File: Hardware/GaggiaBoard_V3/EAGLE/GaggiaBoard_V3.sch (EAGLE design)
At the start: 73 parts, among them IC1 LD117AS33TR, J1 4PIN, J10 PIN262409-1, J11 PIN262409-1, J12 PIN262409-1, J13 PIN262409-1, J2 Vertical Qwiic Connector, J27 6PIN, J5 2PIN, J6 3PIN, J7 3PIN, J8 5PIN, J9 3PIN, K1 AQH213, Q10 600mA/40V, Q11 MOSFET_PCH_DUAL-DMP2240UDM, U1 BLACKPILL, U2 MAX31855K, U5 TXS0102

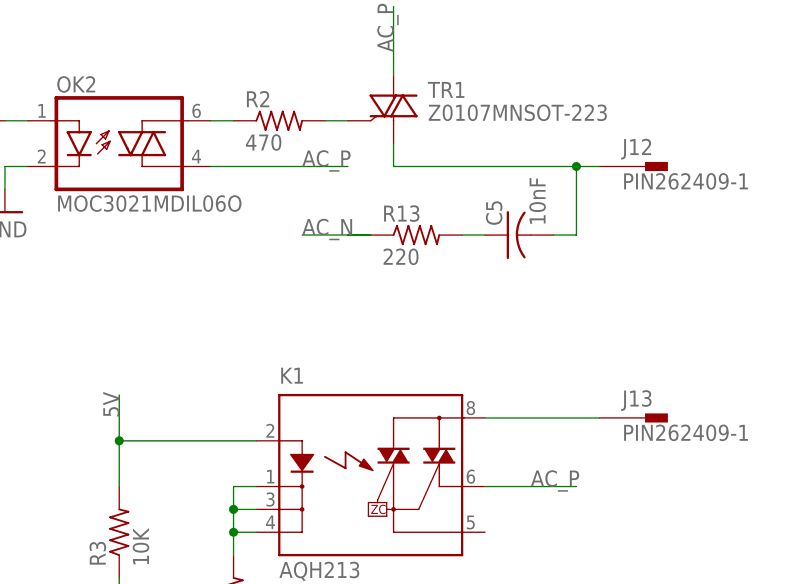
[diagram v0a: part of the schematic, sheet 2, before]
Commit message: snubbers
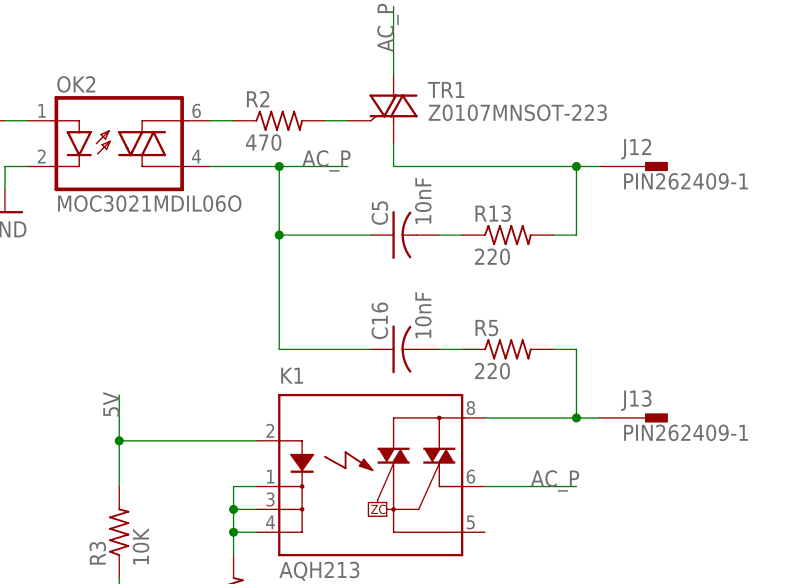
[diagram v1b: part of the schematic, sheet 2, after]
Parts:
- added C16: 10nF, rcl:C-USC1206
- added R5: 220, rcl:R-US_R2512
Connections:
- removed net N$32: C5.1, R13.2
- new net N$15: C16.2, R5.1
- new net N$16: C5.2, R13.1
- net 3WAY: now also R5.2
- net AC_N: no longer R13.1
- net AC_P: now also C16.1, C5.1
- net PUMP_P: now also R13.2; no longer C5.2
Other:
- moved on the sheet: C5, R13
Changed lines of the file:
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@@
 <attribute name="LCSC" value="C98220"/>
+</part>
+<part name="R5" library="rcl" library_urn="urn:adsk.eagle:library:334" deviceset="R-US_" device="R2512" package3d_urn="urn:adsk.eagle:package:23545/2" value="220">
+<spice>
+<pinmapping spiceprefix="R">
+<pinmap gate="G$1" pin="1" pinorder="1"/>
+<pinmap gate="G$1" pin="2" pinorder="2"/>
+</pinmapping>
+</spice>
+<attribute name="LCSC" value="C877859"/>
+</part>
+<part name="C16" library="rcl" library_urn="urn:adsk.eagle:library:334" deviceset="C-US" device="C1206" package3d_urn="urn:adsk.eagle:package:23618/2" value="10nF">
+<spice>
+<pinmapping spiceprefix="C">
+<pinmap gate="G$1" pin="1" pinorder="1"/>
+<pinmap gate="G$1" pin="2" pinorder="2"/>
+</pinmapping>
+</spice>
+<attribute name="LCSC" value="C107192"/>
 </part>
 </parts>
@@
 <instance part="MARK4" gate="G$1" x="243.84" y="27.94" smashed="yes"/>
 <instance part="MARK3" gate="G$1" x="241.3" y="27.94" smashed="yes"/>
-<instance part="R13" gate="G$1" x="208.28" y="109.22" smashed="yes">
-<attribute name="NAME" x="204.47" y="110.7186" size="1.778" layer="95"/>
-<attribute name="VALUE" x="204.47" y="105.918" size="1.778" layer="96"/>
-<attribute name="LCSC" x="208.28" y="109.22" size="1.778" layer="96" display="off"/>
-</instance>
-<instance part="C5" gate="G$1" x="218.44" y="109.22" smashed="yes" rot="R90">
-<attribute name="NAME" x="217.805" y="110.236" size="1.778" layer="95" rot="R90"/>
-<attribute name="VALUE" x="222.631" y="110.236" size="1.778" layer="96" rot="R90"/>
-<attribute name="LCSC" x="218.44" y="109.22" size="1.778" layer="96" rot="R90" display="off"/>
+<instance part="R13" gate="G$1" x="218.44" y="109.22" smashed="yes">
+<attribute name="NAME" x="214.63" y="110.7186" size="1.778" layer="95"/>
+<attribute name="VALUE" x="214.63" y="105.918" size="1.778" layer="96"/>
+<attribute name="LCSC" x="218.44" y="109.22" size="1.778" layer="96" display="off"/>
+</instance>
+<instance part="C5" gate="G$1" x="205.74" y="109.22" smashed="yes" rot="R90">
+<attribute name="NAME" x="205.105" y="110.236" size="1.778" layer="95" rot="R90"/>
+<attribute name="VALUE" x="209.931" y="110.236" size="1.778" layer="96" rot="R90"/>
+<attribute name="LCSC" x="205.74" y="109.22" size="1.778" layer="96" rot="R90" display="off"/>
 </instance>
 <instance part="MARK6" gate="G$1" x="238.76" y="27.94" smashed="yes"/>
@@
 <attribute name="LCSC" x="162.56" y="63.5" size="1.778" layer="96" display="off"/>
 </instance>
+<instance part="R5" gate="G$1" x="218.44" y="96.52" smashed="yes">
+<attribute name="NAME" x="214.63" y="98.0186" size="1.778" layer="95"/>
+<attribute name="VALUE" x="214.63" y="93.218" size="1.778" layer="96"/>
+<attribute name="LCSC" x="218.44" y="96.52" size="1.778" layer="96" display="off"/>
+</instance>
+<instance part="C16" gate="G$1" x="205.74" y="96.52" smashed="yes" rot="R90">
+<attribute name="NAME" x="205.105" y="97.536" size="1.778" layer="95" rot="R90"/>
+<attribute name="VALUE" x="209.931" y="97.536" size="1.778" layer="96" rot="R90"/>
+<attribute name="LCSC" x="205.74" y="96.52" size="1.778" layer="96" rot="R90" display="off"/>
+</instance>
 </instances>
 <busses>
@@
 </segment>
 <segment>
-<label x="195.58" y="109.22" size="1.778" layer="95"/>
-<pinref part="R13" gate="G$1" pin="1"/>
-<wire x1="203.2" y1="109.22" x2="200.66" y2="109.22" width="0.1524" layer="91"/>
-<wire x1="195.58" y1="109.22" x2="203.2" y2="109.22" width="0.1524" layer="91"/>
-</segment>
-<segment>
 <label x="5.08" y="68.58" size="1.778" layer="95"/>
 <wire x1="15.24" y1="68.58" x2="5.08" y2="68.58" width="0.1524" layer="91"/>
@@
 <segment>
 <pinref part="OK2" gate="G$1" pin="A1"/>
-<wire x1="185.42" y1="116.84" x2="200.66" y2="116.84" width="0.1524" layer="91"/>
+<wire x1="185.42" y1="116.84" x2="193.04" y2="116.84" width="0.1524" layer="91"/>
 <label x="195.58" y="116.84" size="1.778" layer="95"/>
+<pinref part="C5" gate="G$1" pin="1"/>
+<wire x1="193.04" y1="116.84" x2="200.66" y2="116.84" width="0.1524" layer="91"/>
+<wire x1="203.2" y1="109.22" x2="193.04" y2="109.22" width="0.1524" layer="91"/>
+<wire x1="193.04" y1="109.22" x2="193.04" y2="116.84" width="0.1524" layer="91"/>
+<junction x="193.04" y="116.84"/>
+<pinref part="C16" gate="G$1" pin="1"/>
+<wire x1="203.2" y1="96.52" x2="193.04" y2="96.52" width="0.1524" layer="91"/>
+<wire x1="193.04" y1="96.52" x2="193.04" y2="109.22" width="0.1524" layer="91"/>
+<junction x="193.04" y="109.22"/>
 </segment>
 <segment>
@@
 <net name="3WAY" class="0">
 <segment>
-<wire x1="228.6" y1="88.9" x2="215.9" y2="88.9" width="0.1524" layer="91"/>
+<wire x1="228.6" y1="88.9" x2="226.06" y2="88.9" width="0.1524" layer="91"/>
 <pinref part="J13" gate="-1" pin="1"/>
 <pinref part="K1" gate="G$1" pin="DS1"/>
+<pinref part="R5" gate="G$1" pin="2"/>
+<wire x1="226.06" y1="88.9" x2="215.9" y2="88.9" width="0.1524" layer="91"/>
+<wire x1="223.52" y1="96.52" x2="226.06" y2="96.52" width="0.1524" layer="91"/>
+<wire x1="226.06" y1="96.52" x2="226.06" y2="88.9" width="0.1524" layer="91"/>
+<junction x="226.06" y="88.9"/>
 </segment>
 </net>
@@
 </segment>
 </net>
-<net name="N$32" class="0">
-<segment>
-<pinref part="C5" gate="G$1" pin="1"/>
-<pinref part="R13" gate="G$1" pin="2"/>
-<wire x1="215.9" y1="109.22" x2="213.36" y2="109.22" width="0.1524" layer="91"/>
-</segment>
-</net>
 <net name="PUMP_P" class="0">
 <segment>
 <pinref part="J12" gate="-1" pin="1"/>
 <wire x1="228.6" y1="116.84" x2="226.06" y2="116.84" width="0.1524" layer="91"/>
+<pinref part="TR1" gate="G$1" pin="A1"/>
 <wire x1="226.06" y1="116.84" x2="205.74" y2="116.84" width="0.1524" layer="91"/>
-<pinref part="C5" gate="G$1" pin="2"/>
+<wire x1="205.74" y1="116.84" x2="205.74" y2="119.38" width="0.1524" layer="91"/>
+<pinref part="R13" gate="G$1" pin="2"/>
 <wire x1="223.52" y1="109.22" x2="226.06" y2="109.22" width="0.1524" layer="91"/>
 <wire x1="226.06" y1="109.22" x2="226.06" y2="116.84" width="0.1524" layer="91"/>
 <junction x="226.06" y="116.84"/>
-<pinref part="TR1" gate="G$1" pin="A1"/>
-<wire x1="205.74" y1="116.84" x2="205.74" y2="119.38" width="0.1524" layer="91"/>
 </segment>
 </net>
@@
 </segment>
 </net>
+<net name="N$15" class="0">
+<segment>
+<pinref part="R5" gate="G$1" pin="1"/>
+<pinref part="C16" gate="G$1" pin="2"/>
+<wire x1="213.36" y1="96.52" x2="210.82" y2="96.52" width="0.1524" layer="91"/>
+</segment>
+</net>
+<net name="N$16" class="0">
+<segment>
+<pinref part="R13" gate="G$1" pin="1"/>
+<pinref part="C5" gate="G$1" pin="2"/>
+<wire x1="213.36" y1="109.22" x2="210.82" y2="109.22" width="0.1524" layer="91"/>
+</segment>
+</net>
